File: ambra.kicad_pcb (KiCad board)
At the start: 2 copper layers, 129.8 x 98.6 mm, 33 parts, among them J1 MJ-4PP-9, SW1 SW_SPDT, U1 ProMicro_r

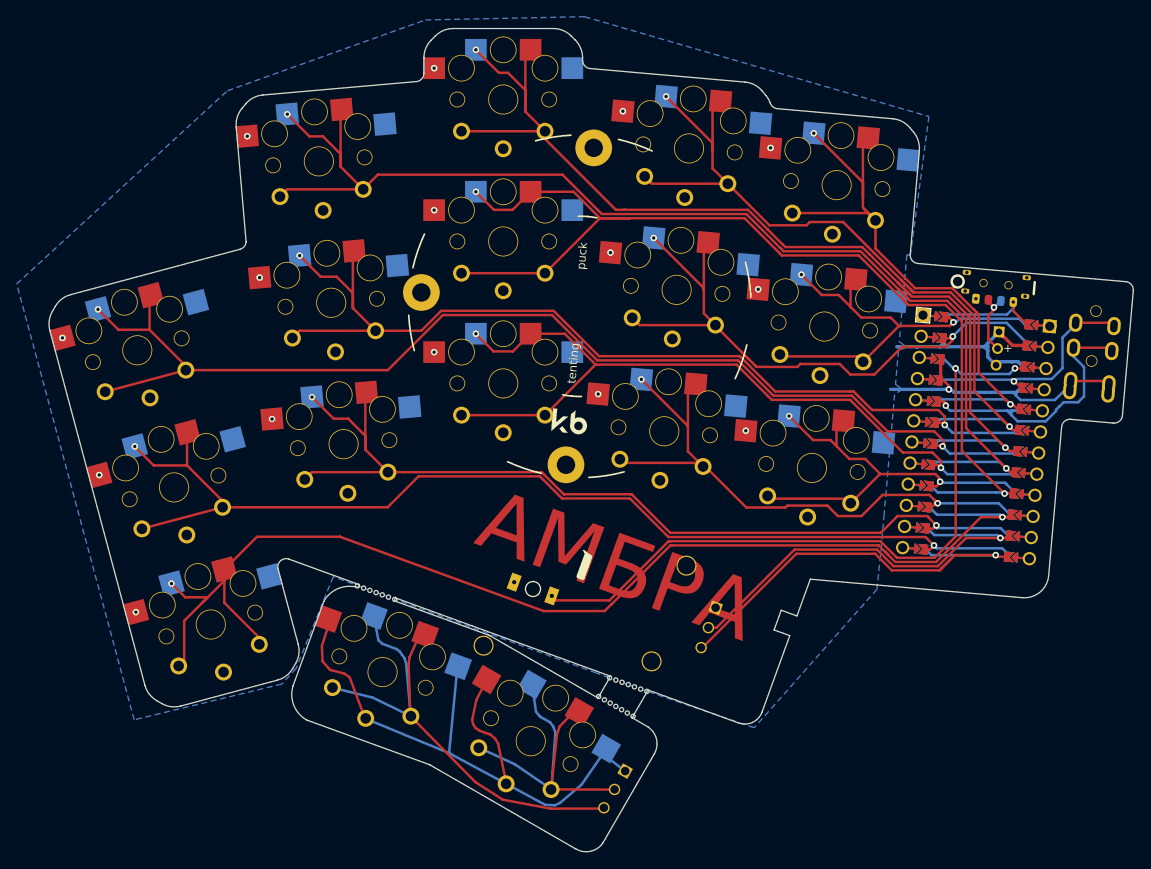
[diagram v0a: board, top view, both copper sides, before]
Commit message: Add files via upload
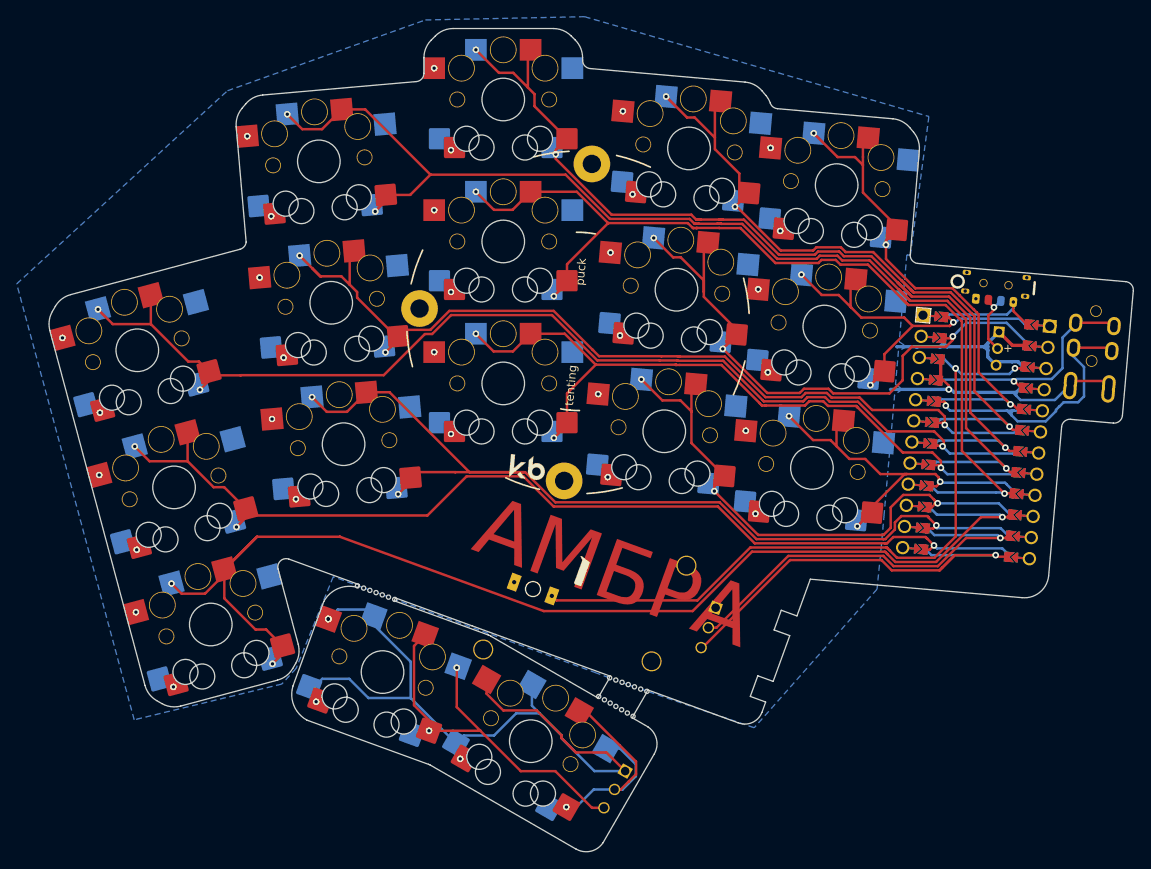
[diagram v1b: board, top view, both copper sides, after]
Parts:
- SWr1c1, SWr1c2, SWr1c3, SWr1c4, SWr1c5, SWr2c1, SWr2c2, SWr2c3, SWr2c4, SWr2c5, SWr3c1, SWr3c2, SWr3c3, SWr3c4, SWr3c5, SWr4c1, SWr4c2: footprint my syms-foots:ChocV1_duplex_hotswap_topor -> my syms-foots:Choc-and-KS33-Hotswap-Choc-1U
- moved REF** 1.94 mm to (156.3, 83.7)
- moved H1 0.46 mm to (145.0, 122.9)
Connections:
- SWr4c1 pad 2: GND2 -> db1
- SWr4c2 pad 2: GND2 -> db2
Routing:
- net GND2: track 75.1 -> 92.3 mm, vias 0 -> 4
- net r1c1: track 73.8 -> 59.6 mm, vias 2 -> 3
- net db2: track 59.7 -> 47.6 mm, vias 0 -> 2
- net r2c3: track 123.1 -> 111.8 mm, vias 2 -> 3
- net r2c4: track 116.6 -> 105.7 mm, vias 2 -> 3
- net r1c3: track 122.4 -> 112.2 mm, vias 2 -> 3
- net db1: track 40.3 -> 30.4 mm, vias 0 -> 1
- net r1c2: track 92.9 -> 83.6 mm, vias 2 -> 3
- net r1c4: track 142.8 -> 133.9 mm, vias 2 -> 3
- net r1c5: track 138.3 -> 129.6 mm, vias 2 -> 3
- net r2c5: track 128.0 -> 119.9 mm, vias 2 -> 3
- net r3c3: track 93.3 -> 86.2 mm, vias 2 -> 3
- net r2c1: track 51.5 -> 44.6 mm, vias 2 -> 3
- net r3c1: track 48.3 -> 42.4 mm, vias 2 -> 3
- net r2c2: track 74.9 -> 70.1 mm, vias 2 -> 3
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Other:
- outline, holes or cut-outs redrawn
